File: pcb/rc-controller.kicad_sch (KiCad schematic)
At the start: 3 parts, among them M1 Motor_DC, M2 Motor_DC, U1 STM32F401RCTx

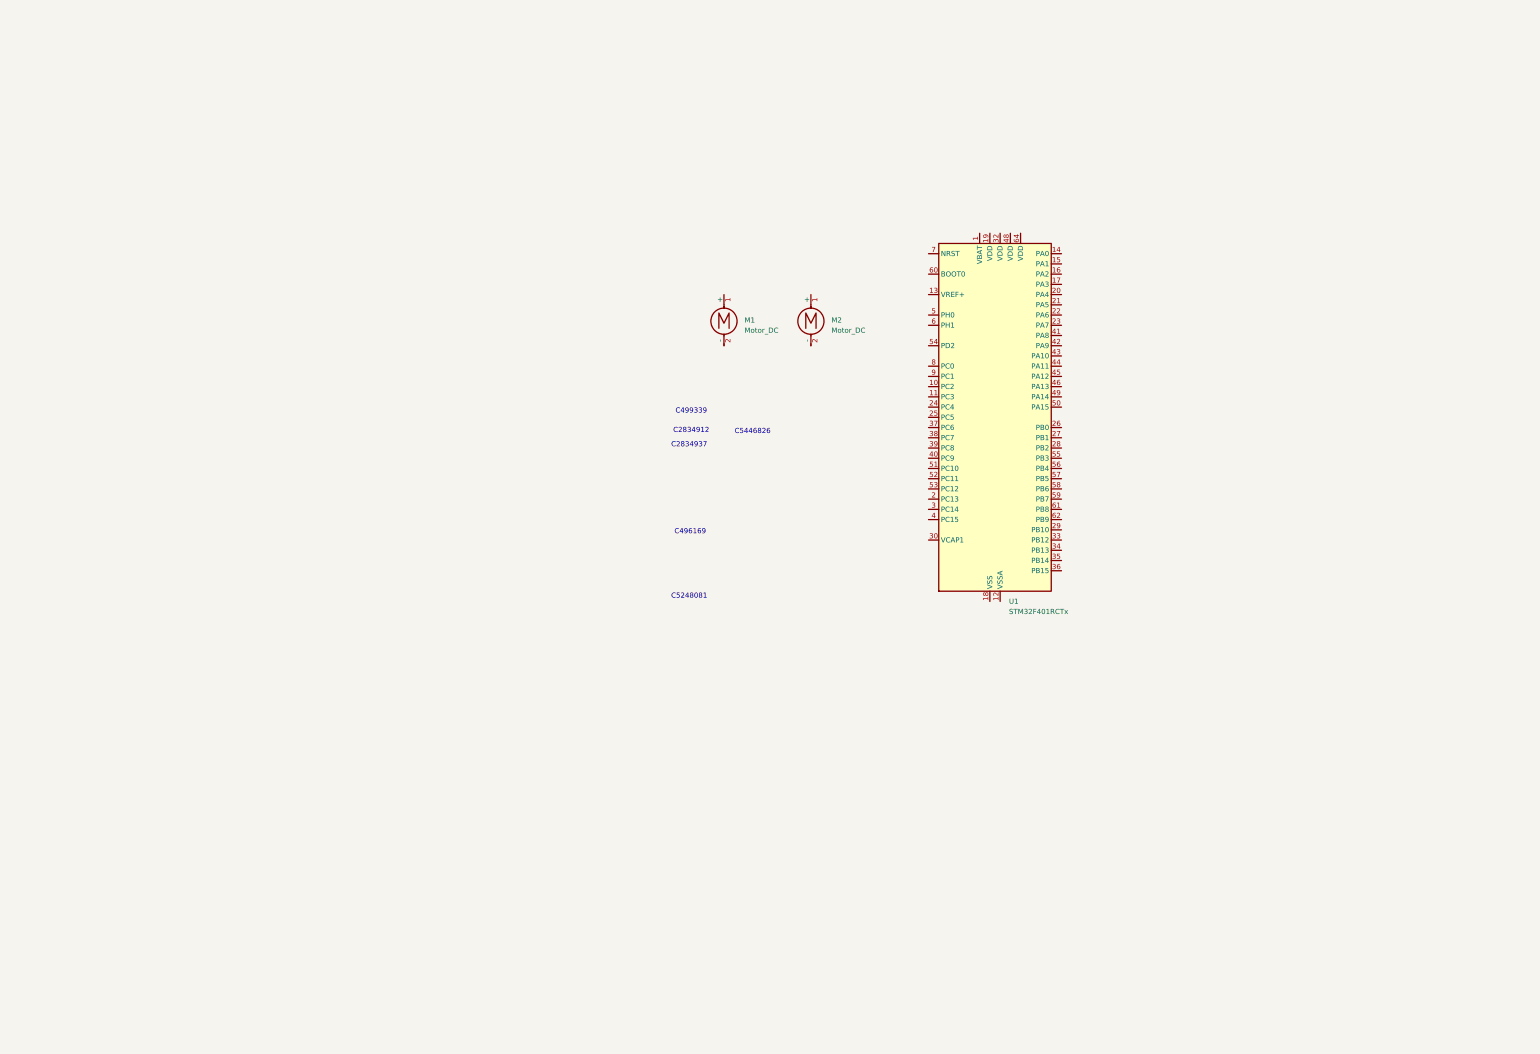
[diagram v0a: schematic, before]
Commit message: Update .gitignore
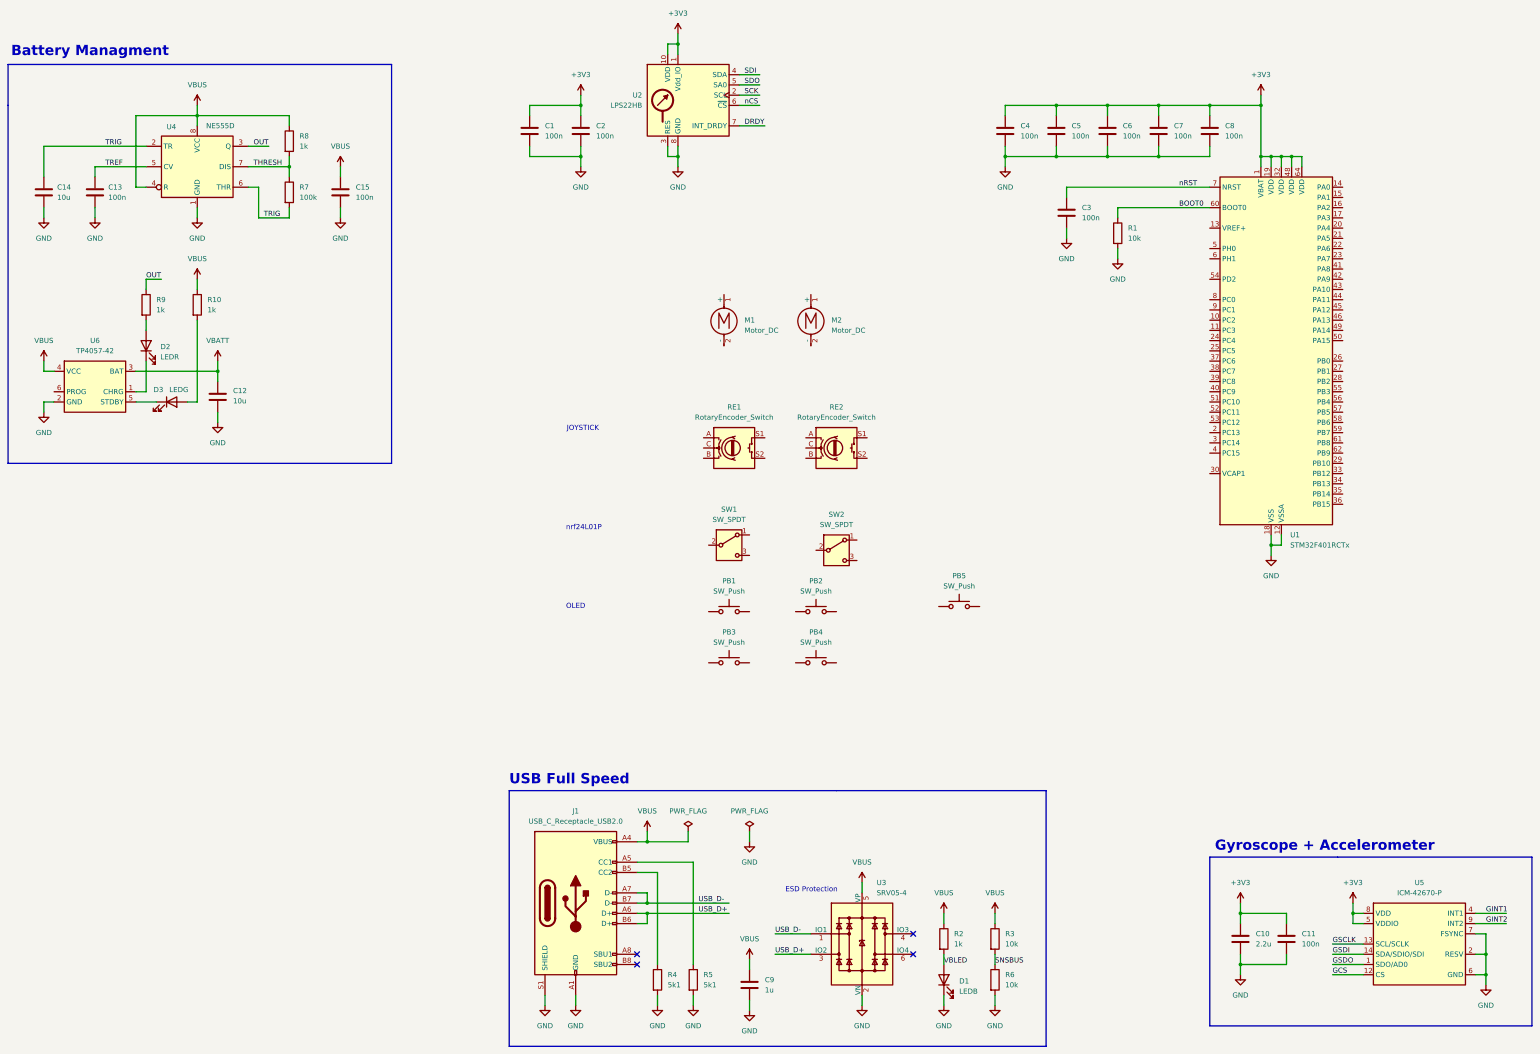
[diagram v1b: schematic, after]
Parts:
- added C1, C11, C2: 100n, Capacitor_SMD:C_0402_1005Metric, symbol Device:C
- added C10: 2.2u, Capacitor_SMD:C_0603_1608Metric, symbol Device:C
- added C12, C14: 10u, symbol Device:C
- added C13, C15, C3, C4, C5, C6, C7, C8: 100n, symbol Device:C
- added C9: 1u, Capacitor_SMD:C_0402_1005Metric, symbol Device:C
- added D1: LEDB, LED_SMD:LED_0603_1608Metric, symbol Device:LED
- added D2: LEDR, symbol Device:LED
- added D3: LEDG, symbol Device:LED
- added J1: USB_C_Receptacle_USB2.0, Connector_USB:USB_C_Receptacle_GCT_USB4105-xx-A_16P_TopMnt_Horizontal, symbol Connector:USB_C_Receptacle_USB2.0
- added PB1, PB2, PB3, PB4, PB5: SW_Push, symbol Switch:SW_Push
- added R1: 10k, symbol Device:R
- added R10, R2, R9: 1k, Resistor_SMD:R_0402_1005Metric, symbol Device:R
- added R3, R6: 10k, Resistor_SMD:R_0402_1005Metric, symbol Device:R
- added R4, R5: 5k1, Resistor_SMD:R_0402_1005Metric, symbol Device:R
- added R7: 100k, symbol Device:R
- added R8: 1k, symbol Device:R
- added RE1, RE2: RotaryEncoder_Switch, symbol Device:RotaryEncoder_Switch
- added SW1, SW2: SW_SPDT, symbol Switch:SW_SPDT
- added U2: LPS22HB, Package_LGA:ST_HLGA-10_2x2mm_P0.5mm_LayoutBorder3x2y, symbol Sensor_Pressure:LPS22HB
- added U3: SRV05-4, Package_TO_SOT_SMD:SOT-23-6, symbol Power_Protection:SRV05-4
- added U4: NE555D, Package_SO:SOIC-8_3.9x4.9mm_P1.27mm, symbol Timer:NE555D
- added U5: ICM-42670-P, Package_LGA:LGA-14_3x2.5mm_P0.5mm_LayoutBorder3x4y, symbol MySymbols:ICM-42670-P
- added U6: TP4057-42, Package_TO_SOT_SMD:TSOT-23-6, symbol User_Symbols:TP4057-42
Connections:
- net +3V3: now reaches U1.1 (VBAT)
- net +3V3: now also U1.19 (VDD), U1.32 (VDD), U1.48 (VDD), U1.64 (VDD), C1.1, C10.1, C11.1, C2.1, C4.1, C5.1, C6.1, C7.1, C8.1, U2.1 (Vdd_IO), U2.10 (VDD), U5.5 (VDDIO), U5.8 (VDD)
- net GND: now reaches U1.12 (VSSA)
- net GND: now also U1.18 (VSS), U1.31 (VSS), U1.47 (VSS), U1.63 (VSS), C1.2, C10.2, C11.2, C12.2, C13.2, C14.2, C15.2, C2.2, C3.2, C4.2, C5.2, C6.2, C7.2, C8.2, C9.2, D1.1 (K), J1.A1 (GND), J1.A12 (GND), J1.B1 (GND), J1.B12 (GND), J1.S1 (SHIELD), R1.2, R4.2, R5.2, R6.2, U2.3 (RES), U2.8 (GND), U2.9 (GND), U3.2 (VN), U4.1 (GND), U5.10 (RESV), U5.11 (RESV), U5.2 (RESV), U5.3 (RESV), U5.6 (GND), U5.7 (FSYNC), U6.2 (GND)
- net BOOT0: now reaches U1.60 (BOOT0)
- net BOOT0: now also R1.1
- net nRST: now reaches U1.7 (NRST)
- net nRST: now also C3.1
- new net: D2.1 (K), U6.1 (CHRG)
- new net: D2.2 (A), R9.2
- new net: D3.2 (A), R10.2
- new net: J1.A5 (CC1), R5.1
- new net: D3.1 (K), U6.5 (STDBY)
- new net: J1.B5 (CC2), R4.1
- new net DRDY: U2.7 (INT_DRDY)
- new net GCS: U5.12 (CS)
- new net GINT1: U5.4 (INT1)
- new net GINT2: U5.9 (INT2)
- new net GSCLK: U5.13 (SCL/SCLK)
- new net GSDI: U5.14 (SDA/SDIO/SDI)
- new net GSDO: U5.1 (SDO/AD0)
- new net OUT: R9.1, U4.3 (Q)
- new net SCK: U2.2 (SCL)
- new net SDI: U2.4 (SDA)
- new net SDO: U2.5 (SA0)
- new net SNSBUS: R3.2, R6.1
- new net THRESH: R7.1, R8.2, U4.7 (DIS)
- new net TREF: C13.1, U4.5 (CV)
- new net TRIG: C14.1, R7.2, U4.2 (TR), U4.6 (THR)
- new net USB_D+: J1.A6 (D+), J1.B6 (D+), U3.3 (IO2)
- new net USB_D-: J1.A7 (D-), J1.B7 (D-), U3.1 (IO1)
- new net VBATT: C12.1, U6.3 (BAT)
- new net VBLED: D1.2 (A), R2.2
- new net VBUS: C15.1, C9.1, J1.A4 (VBUS), J1.A9 (VBUS), J1.B4 (VBUS), J1.B9 (VBUS), R10.1, R2.1, R3.1, R8.1, U3.5 (VP), U4.4 (R), U4.8 (VCC), U6.4 (VCC)
- new net nCS: U2.6 (~{CS})
- no-connect marks 0 -> 4
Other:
- note added: "Battery Managment"
- note added: "ESD Protection"
- note added: "Gyroscope + Accelerometer"
- note added: "JOYSTICK"
- note added: "OLED"
- note added: "USB Full Speed"
- note added: "nrf24L01P"
- note removed: "C2834912"
- note removed: "C2834937"
- note removed: "C496169"
- note removed: "C499339"
- note removed: "C5248081"
- note removed: "C5446826"
- moved on the sheet: U1
